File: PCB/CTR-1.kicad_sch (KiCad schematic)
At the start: 44 parts, among them J1 Conn_Coaxial, J2 JTAG, J3 UART, SW1 RST, SW2 BOOT, U1 ESP32-S3, U2 W25Q128JVP, U3 ESP-PSRAM64H, Y1 32kHz, Y2 40MHz

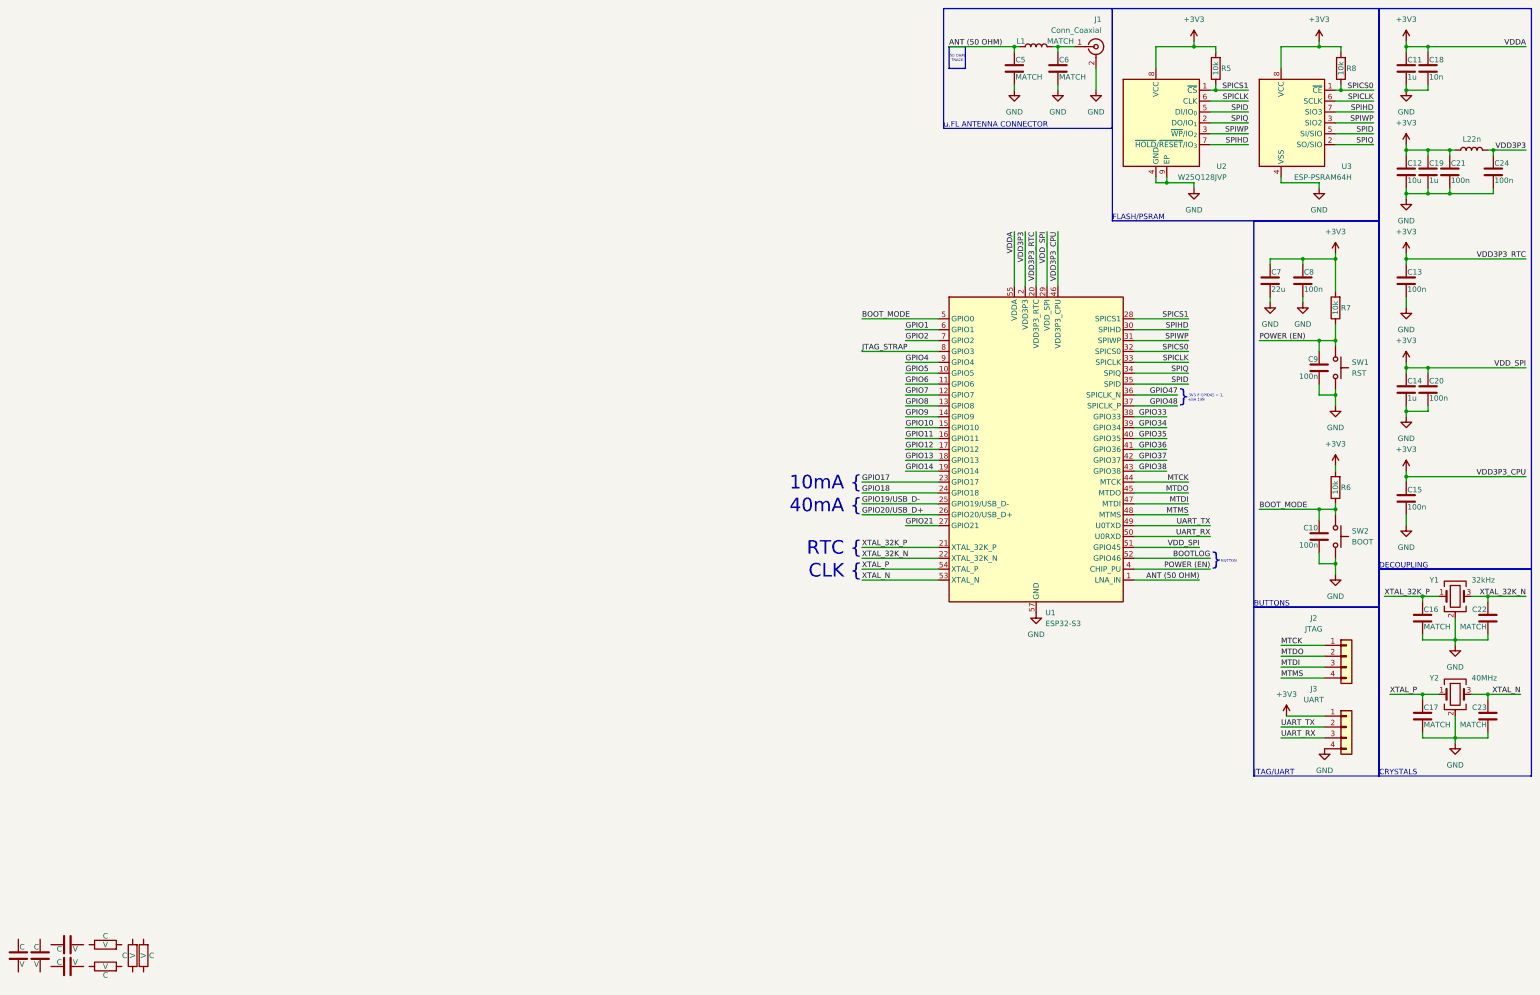
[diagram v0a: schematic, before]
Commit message: schematic polish
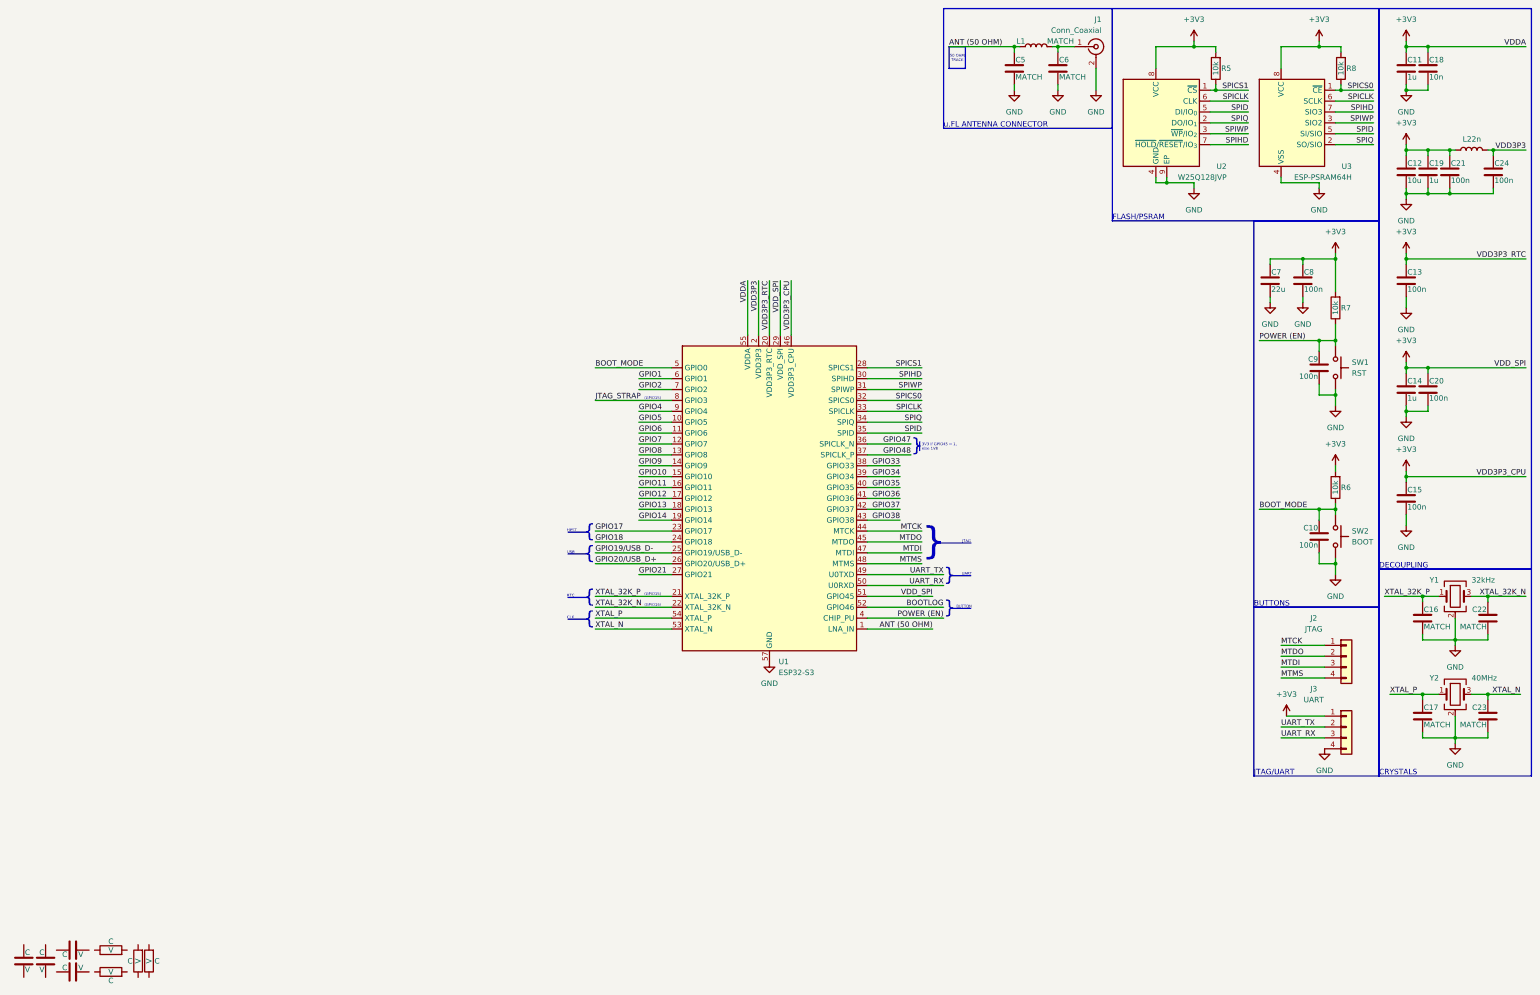
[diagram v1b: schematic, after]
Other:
- note added: "(GPIO15)"
- note added: "(GPIO16)"
- note added: "CLK"
- note added: "HPST"
- note added: "JTAG"
- note added: "RTC"
- note added: "UART"
- note added: "USB"
- note added: "{"
- note removed: "10mA {"
- note removed: "40mA {"
- note removed: "CLK {"
- note removed: "RTC {"
- moved on the sheet: C, U1
